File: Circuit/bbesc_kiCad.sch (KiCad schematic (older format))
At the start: 79 parts, among them J1 CONN_01X02, J10 CONN_01X01, J11 CONN_01X01, J12 CONN_01X01, J13 CONN_01X01, J14 CONN_01X01, J15 CONN_01X02, J16 CONN_01X02, J17 CONN_01X01, J18 CONN_01X01, J19 CONN_01X01, J2 CONN_01X06, J3 CONN_01X06, J4 CONN_01X06, J5 CONN_01X02, J6 CONN_01X02, J7 CONN_01X01, J8 CONN_01X01, J9 RJ45, Q1 Q_NMOS_GDS, Q2 Q_NMOS_GDS, Q3 Q_NMOS_GDS, Q4 Q_NMOS_GDS, Q5 Q_NMOS_GDS, Q6 Q_NMOS_GDS, U1 teensy_3-2, U2 IR2101, U3 IR2101, U4 IR2101, U5 LM324N, U6 LM7805

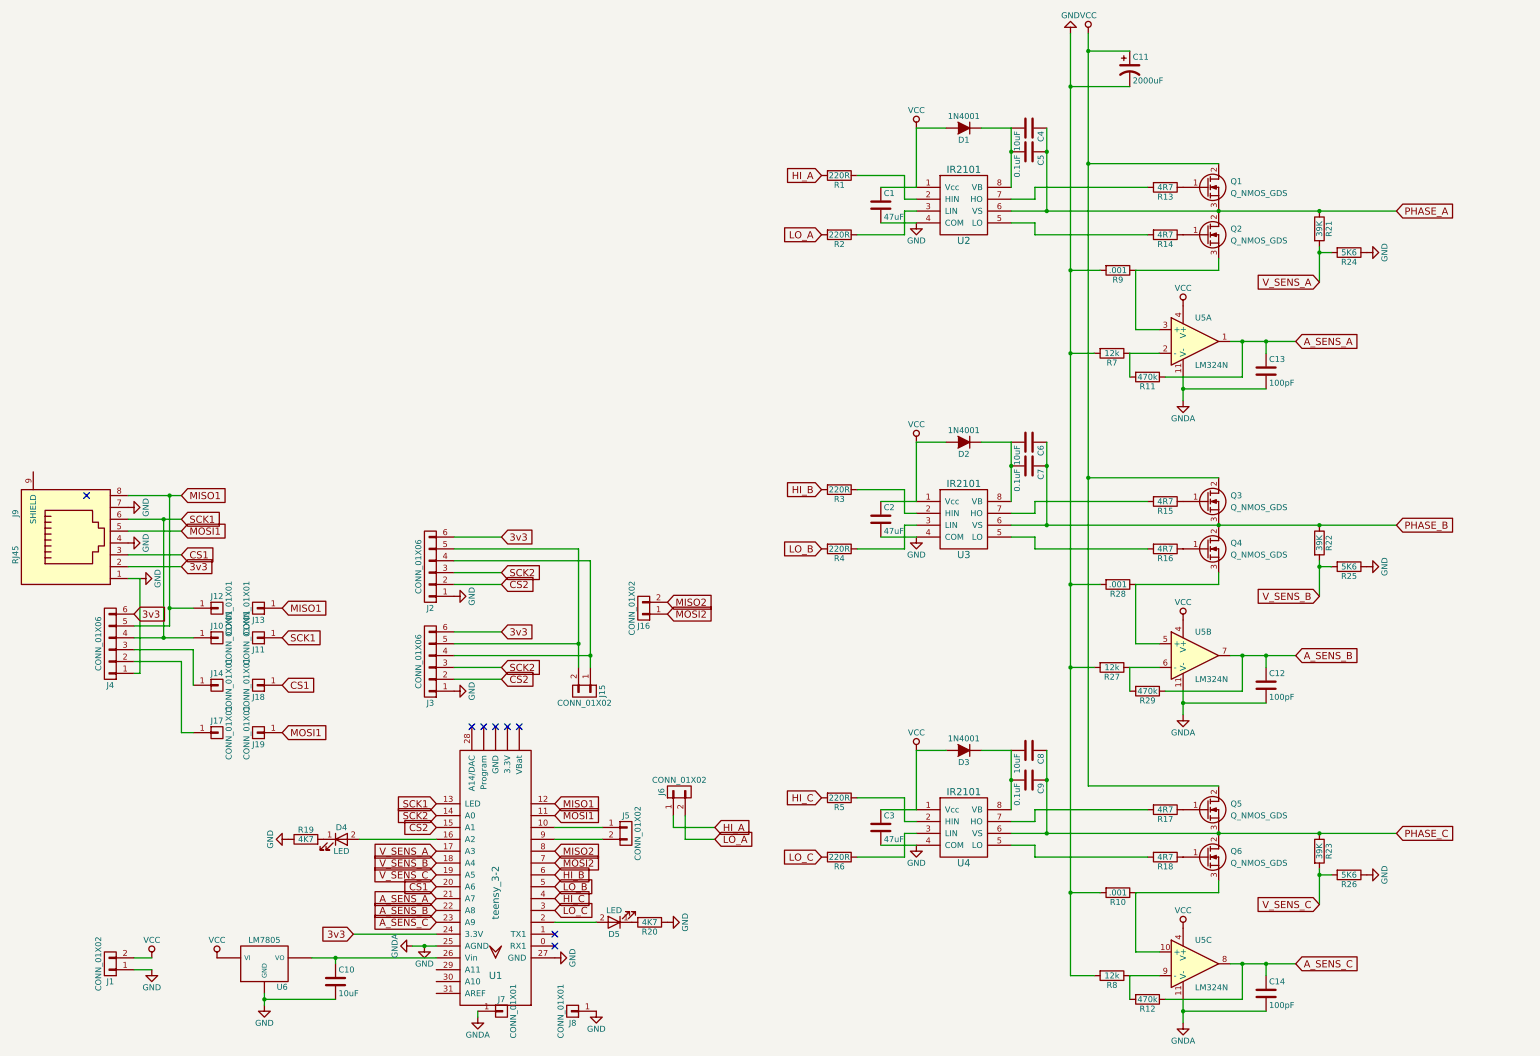
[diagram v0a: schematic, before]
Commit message: circuit for fab, foc bones
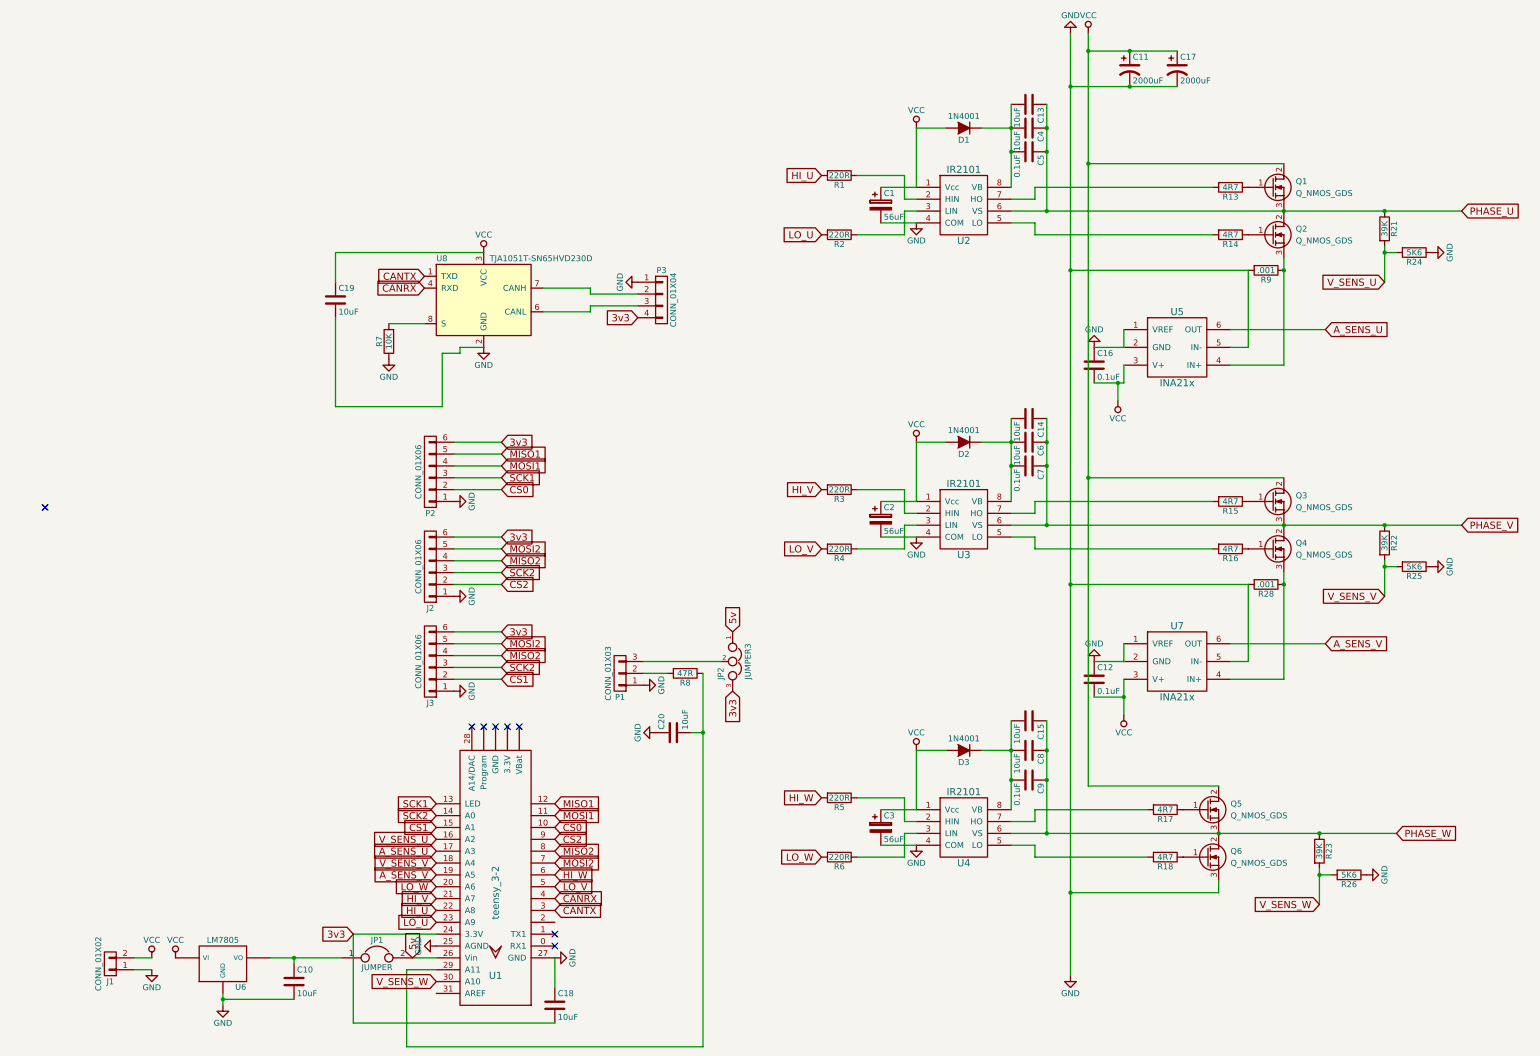
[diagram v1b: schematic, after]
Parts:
- removed C1, C2, C3: 47uF, Capacitors_SMD:C_1206_HandSoldering, symbol C
- removed D4, D5: LED, LEDs:LED_1206, symbol LED-RESCUE-bbesc_kiCad
- removed J10, J11, J12, J13, J14, J17, J18, J19, J7, J8: CONN_01X01, Pin_Headers:Pin_Header_Straight_1x01_Pitch2.54mm, symbol CONN_01X01
- removed J15, J16, J5, J6: CONN_01X02, Pin_Headers:Pin_Header_Straight_1x02_Pitch2.54mm, symbol CONN_01X02
- removed J4: CONN_01X06, Pin_Headers:Pin_Header_Straight_1x06_Pitch2.54mm, symbol CONN_01X06
- removed J9: RJ45, Connectors:RJ45_8, symbol RJ45
- removed R10: .001, R_SHUNT_3920:R_2816_HandSoldering, symbol R
- removed R11, R12, R29: 470k, Resistors_SMD:R_1206_HandSoldering, symbol R
- removed R19, R20: 4K7, Resistors_SMD:R_1206_HandSoldering, symbol R
- removed R27: 12k, Resistors_SMD:R_1206_HandSoldering, symbol R
- removed U5: LM324N, Housings_DIP:DIP-14_W7.62mm_Socket_LongPads, symbol LM324N
- added C1, C2, C3: 56uF, Capacitors_SMD:CP_Elec_6.3x7.7, symbol CP
- added C15, C18, C19, C20: 10uF, Capacitors_SMD:C_1206_HandSoldering, symbol C
- added C16: 0.1uF, Capacitors_SMD:C_1206_HandSoldering, symbol C
- added C17: 2000uF, Capacitors_ThroughHole:CP_Radial_D13.0mm_P5.00mm, symbol CP1
- added JP1: JUMPER, Pin_Headers:Pin_Header_Straight_1x02_Pitch2.54mm, symbol JUMPER
- added JP2: JUMPER3, Pin_Headers:Pin_Header_Straight_1x03_Pitch2.54mm, symbol JUMPER3
- added P1: CONN_01X03, Pin_Headers:Pin_Header_Straight_1x03_Pitch2.54mm, symbol CONN_01X03
- added P2: CONN_01X06, Pin_Headers:Pin_Header_Straight_1x06_Pitch2.54mm, symbol CONN_01X06
- added P3: CONN_01X04, Pin_Headers:Pin_Header_Straight_1x04_Pitch2.54mm, symbol CONN_01X04
- added U5, U7: INA21x, TO_SOT_Packages_SMD:SOT-363_SC-70-6_Handsoldering, symbol INA21x
- added U8: TJA1051T-SN65HVD230D, Housings_SOIC:SOIC-8_3.9x4.9mm_Pitch1.27mm, symbol TJA1051T
- C11: footprint Capacitors_THT:CP_Radial_D16.0mm_P7.50mm -> Capacitors_ThroughHole:CP_Radial_D13.0mm_P5.00mm
- C12: value 100pF -> 0.1uF
- C13, C14: value 100pF -> 10uF
- R7: value 12k -> 10K
- R8: value 12k -> 47R
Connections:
- net HI_A is gone; now on net HI_U: R1.2
- net LO_A is gone; now on net LO_U: R2.2
- net 3v3: now also C18.2, JP2.3, P2.6 (P6), P3.4 (P4)
- net CS1: now also J3.2 (P2), U1.15 (A1); no longer U1.20 (A6)
- net CS2: now also U1.9; no longer J3.2 (P2), U1.15 (A1)
- net GND: now also C12.1, Q6.3 (S), R7.1, C1.2, C16.1, C17.2, C18.1, C19.2, C2.2, C20.1, C3.2, P1.1 (P1), P2.1 (P1), P3.1 (P1), U5.1 (VREF), U5.2 (GND), U5.5 (IN-), U7.1 (VREF), U7.2 (GND), U7.5 (IN-), U8.2 (GND); no longer C12.2, C13.2, C14.2, R7.2, R8.2
- net MISO1: now also P2.5 (P5)
- net MISO2: now also J2.4 (P4), J3.4 (P4)
- net MOSI1: now also P2.4 (P4)
- net MOSI2: now also J2.5 (P5), J3.5 (P5)
- net SCK1: now also P2.3 (P3)
- net VCC: now also C12.2, C1.1, C16.2, C17.1, C19.1, C2.1, C3.1, U5.3 (V+), U7.3 (V+), U8.3 (VCC)
- net at C8.2, C9.2, D3.1 (K)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: now also C15.2
- net at R8.1: now also U1.29 (A11), C20.2
- net at Q4.3 (S), R28.1: now also U7.4 (IN+)
- net at C6.2, C7.2, D2.1 (K)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: now also C14.2
- net at Q2.3 (S), R9.1: now also U5.4 (IN+)
- net at C4.2, C5.2, D1.1 (K)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: now also C13.2
- net CS0: now reaches U1.10
- net CS0: now also P2.2 (P2)
- net V_SENS_U: now reaches U1.16 (A2)
- net V_SENS_U: now also R21.2, R24.2
- net at C10.1, U6.3 (VO): now also JP1.1; no longer U1.26 (Vin)
- net V_SENS_W: now reaches U1.30 (A10)
- net V_SENS_W: now also R23.2, R26.2
- net A_SENS_A renamed HI_V
- net HI_V: now also R3.2; no longer C13.1
- net A_SENS_B renamed HI_U
- net HI_U: no longer C12.1
- net A_SENS_C renamed LO_U
- net LO_U: no longer C14.1
- net HI_B renamed HI_W
- net HI_W: now also R5.2; no longer R3.2
- net HI_C renamed CANRX
- net CANRX: now also U8.4 (RXD); no longer R5.2
- net LO_B renamed LO_V
- net LO_C renamed CANTX
- net CANTX: now also U8.1 (TXD); no longer R6.2
- net PHASE_A renamed PHASE_U
- net PHASE_U: now also C13.1
- net PHASE_B renamed PHASE_V
- net PHASE_V: now also C14.1
- net PHASE_C renamed PHASE_W
- net PHASE_W: now also C15.1
- removed net V_SENS_A: R21.2, R24.2, U1.17 (A3)
- net V_SENS_B renamed V_SENS_V
- removed net V_SENS_C: R23.2, R26.2, U1.19 (A5)
- new net: P1.2 (P2), R8.2
- new net: JP2.2, P1.3 (P3)
- new net: P3.3 (P3), U8.6 (CANL)
- new net: P3.2 (P2), U8.7 (CANH)
- new net: R7.2, U8.8 (S)
- new net 5v: JP1.2, JP2.1, U1.26 (Vin)
- new net A_SENS_U: U1.17 (A3), U5.6 (OUT)
- new net A_SENS_V: U1.19 (A5), U7.6 (OUT)
- new net LO_W: R6.2, U1.20 (A6)
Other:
- moved on the sheet: C10, C12, Q1, Q2, Q3, Q4, R13, R14, R15, R16, R21, R22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

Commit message: board v0.2
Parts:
- removed C1, C2, C3: 56uF, Capacitors_SMD:CP_Elec_6.3x7.7, symbol CP
- removed C8: 10uF, Capacitors_SMD:C_1206_HandSoldering, symbol C
- removed D1, D3: 1N4001, Diodes_SMD:D_SMA_Handsoldering, symbol D
- removed R1, R2: 220R, Resistors_SMD:R_1206_HandSoldering, symbol R
- removed R22: 39K, Resistors_SMD:R_1206_HandSoldering, symbol R
- removed R28: .001, R_SHUNT_3920:R_2816_HandSoldering, symbol R
- removed U2, U3, U4: IR2101, Housings_DIP:DIP-8_W7.62mm_Socket_LongPads, symbol IR2101
- removed U5, U7: INA21x, TO_SOT_Packages_SMD:SOT-363_SC-70-6_Handsoldering, symbol INA21x
- removed U6: LM7805, TO_SOT_Packages_THT:TO-220_Horizontal, symbol LM7805-RESCUE-bbesc_kiCad
- added C11: 22nF, Capacitors_SMD:C_1206_HandSoldering, symbol C
- added C17: 100nF, Capacitors_SMD:C_1206_HandSoldering, symbol C
- added C18, C19, C20: 220nF, Capacitors_SMD:C_1206_HandSoldering, symbol C
- added C21, C22: 2.2nF, Capacitors_SMD:C_1206_HandSoldering, symbol C
- added C24: 100uF, Capacitors_SMD:CP_Elec_6.3x7.7, symbol CP1
- added C26, C27, C28, C29, C30, C31: 10uF, Capacitors_SMD:C_1206_HandSoldering, symbol C
- added D1: DIODESCH, Diodes_SMD:D_SMA_Handsoldering, symbol D_Schottky
- added JP2: JUMPER, Pin_Headers:Pin_Header_Straight_1x02_Pitch2.54mm, symbol JUMPER
- added L1: 22uH, Inductors:Inductor_Taiyo-Yuden_NR-40xx_HandSoldering, symbol INDUCTOR
- added P4: CONN_01X04, Pin_Headers:Pin_Header_Straight_1x04_Pitch2.54mm, symbol CONN_01X04
- added R10: 1M, Resistors_SMD:R_1206_HandSoldering, symbol R
- added R11, R12, R13, R14: 100R, Resistors_SMD:R_1206_HandSoldering, symbol R
- added R17, R29: 39k, Resistors_SMD:R_1206_HandSoldering, symbol R
- added R18, R24: SHNT, R_SHUNT_3920:R_SHUNT_3920, symbol SHNT
- added R30: 39K, Resistors_SMD:R_1206_HandSoldering, symbol R
- added R31: 5K6, Resistors_SMD:R_1206_HandSoldering, symbol R
- added R7: 3k3, Resistors_SMD:R_1206_HandSoldering, symbol R
- added R8: 15k, Resistors_SMD:R_1206_HandSoldering, symbol R
- added U3: DRV_8302, HTSSOP-56:TSSOP-56_6.1x14mm_Pitch0.5mm, symbol DRV_8302
- C10, C4: value 10uF -> 2.2uF
- C12, C16: value 0.1uF -> 10uF
- C5, C7: value 0.1uF -> 2.2uF
- C6: value 10uF -> 120pF
- C9: value 0.1uF -> 6.8nF
- D2: value 1N4001 -> TVS 5v
- Q1, Q2, Q3, Q4, Q5, Q6: footprint TO-251_IPAK_Slammed:TO-251_IPAK_Vertical -> HTO-252:TO-252-2
- R23: value 39K -> 39k
- R25: value 5K6 -> 39K
- R3: value 220R -> 18k
- R4, R6: value 220R -> 3k3
- R5: value 220R -> 10k
- R9: value .001 -> 220k; footprint R_SHUNT_3920:R_2816_HandSoldering -> Resistors_SMD:R_1206_HandSoldering
- renumbered C19 to C1, C18 to C2, C11 to C23, C17 to C25, C20 to C3, J2 to J1, J3 to J2, J1 to J3, JP2 to JP3, P2 to P1, P1 to P2, R7 to R1, R13 to R15, R14 to R16, R21 to R19, R8 to R2, R24 to R20, R15 to R21, R16 to R22, R17 to R27, R18 to R28, U8 to U1, U1 to U2
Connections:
- net 3v3: now also P4.4 (P4)
- net 5v: now also D2.1 (K), JP1.1, R3.2, R5.2, C24.1, L1.1; no longer JP1.2, U2.26 (Vin)
- net A_SENS_U: now also U3.25 (SO1)
- net A_SENS_V: now also U3.26 (SO2)
- net CS1: now also JP2.2; no longer U2.15 (A1)
- net GND: now also C12.2, C13.2, C14.2, C15.2, C4.2, C5.2, C6.2, C7.2, C9.2, D2.2 (A), Q2.3 (S), R20.2, R26.2, R4.1, R6.1, C24.2, C26.2, C27.2, C28.2, C29.2, C30.2, C31.2, D1.2 (A), P4.1 (P1), R10.1, R17.1, R18.2, R24.2, R31.2, R7.1, U3.28 (AGND), U3.44 (SL_A), U3.57 (GND); no longer C12.1, Q6.3 (S), R20.1, R25.1, R26.1
- net PHASE_U: now also C18.1, U3.46 (SH_A); no longer C13.1, C4.1, C5.1
- net PHASE_V: now also R25.1, C19.1, U3.41 (SH_B); no longer C14.1, C6.1, C7.1
- net PHASE_W: now also C20.1, R30.1, U3.36 (SH_C); no longer C15.1, C9.1, R23.1
- net VCC: now also C12.1, C13.1, C14.1, C15.1, C26.1, C27.1, C28.1, C29.1, C30.1, C31.1, U3.29 (PVDD1), U3.53 (PVDD2), U3.54 (PVDD2); no longer C12.2, D2.2 (A)
- net V_SENS_U: now also R20.1, U2.30 (A10); no longer R20.2, U2.16 (A2)
- net V_SENS_V: now also R26.1
- net V_SENS_W: now also U2.16 (A2), R30.2, R31.1; no longer R23.2, R26.2, U2.30 (A10)
- net at Q6.1 (G), R28.1: now also R29.2
- net at R5.1: now also U3.10 (GAIN), U3.9 (M_OC)
- net DRV_LO_W: now reaches R28.2
- net DRV_LO_W: now also U3.35 (GL_C)
- net DRV_HI_W: now reaches R27.2
- net DRV_HI_W: now also U3.37 (GH_C)
- net at Q4.1 (G), R22.1: now also R23.2
- net H_V_LO: now reaches Q4.3 (S)
- net H_V_LO: now also R23.1, R18.1, U3.39 (SL_B)
- net at R3.1: now also R4.2, U3.3 (VSENS)
- net DRV_LO_V: now reaches R22.2
- net DRV_LO_V: now also U3.40 (GL_B)
- net DRV_HI_V: now reaches R21.2
- net DRV_HI_V: now also U3.42 (GH_B)
- net at R9.1: now also U3.1 (RT_CLK); no longer Q2.3 (S)
- net at Q2.1 (G), R16.1: now also R17.2
- net DRV_LO_U: now reaches R16.2
- net DRV_LO_U: now also U3.45 (GL_A)
- net DRV_HI_U: now reaches R15.2
- net DRV_HI_U: now also U3.47 (GH_A)
- net EN_GATE: now reaches U2.2
- net EN_GATE: now also U3.16 (EN_GATE)
- net DRV_FAULT: now reaches U2.28 (A14/DAC)
- net DRV_FAULT: now also U3.6 (nFAULT)
- net SIMPLE_INPUT: now reaches C3.2, R2.1, U2.29 (A11)
- net MC_AREF: now reaches U2.31 (AREF)
- net MC_AREF: now also U3.24 (REF)
- net at C10.1: now also U3.27 (AVDD); no longer JP1.1
- net at P3.3 (P3), U1.6 (CANL): now also P4.3 (P3)
- net at P3.2 (P2), U1.7 (CANH): now also P4.2 (P2)
- net HI_U renamed MC_HI_U
- net MC_HI_U: now also U3.17 (INH_A)
- net HI_V renamed MC_HI_V
- net MC_HI_V: now also U3.19 (INH_B); no longer R3.2
- net HI_W renamed MC_HI_W
- net MC_HI_W: now also U3.21 (INH_C); no longer R5.2
- net LO_U renamed MC_LO_U
- net MC_LO_U: now also U3.18 (INL_A)
- net LO_V renamed MC_LO_V
- net MC_LO_V: now also U3.20 (INL_B); no longer R4.2
- net LO_W: no longer names the net of R6.2
- net LO_W: now also U3.7 (DTC); no longer U2.20 (A6)
- new net: JP1.2, U2.26 (Vin)
- new net: C4.1, C5.1, U3.11 (OC_ADJ), U3.23 (DVDD)
- new net: C7.1, U3.13 (GVDD)
- new net: C11.1, U3.14 (CP1)
- new net: C11.2, U3.15 (CP2)
- new net: C6.1, R8.1, U3.2 (COMP)
- new net: C22.1, R14.2, U3.30 (SP2)
- new net: C22.2, R13.2, U3.31 (SN2)
- new net: C21.1, R12.2, U3.32 (SP1)
- new net: C21.2, R11.2, U3.33 (SN1)
- new net: C20.2, U3.38 (BST_C)
- new net: C19.2, U3.43 (BST_B)
- new net: C18.2, U3.48 (BST_A)
- new net: R10.2, U3.49 (BIAS)
- new net: C17.1, D1.1 (K), L1.2, U3.50 (PH), U3.51 (PH)
- new net: C17.2, U3.52 (BST_BK)
- new net: R7.2, U3.8 (M_PWM)
- new net: C9.1, R8.2
- new net DC_CAL: JP2.1, U2.15 (A1), U3.12 (DC_CAL)
- new net H_W_LO: Q6.3 (S), R24.1, R29.1, U3.34 (SL_C)
- new net MC_LO_W: U2.20 (A6), U3.22 (INL_C)
- new net SHNT_V_HI: R13.1, R18.3
- new net SHNT_V_LO: R14.1, R18.4
- new net SHNT_W_HI: R11.1, R24.3
- new net SHNT_W_LO: R12.1, R24.4
- no-connect marks 8 -> 11
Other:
- moved on the sheet: C1, C2, C23, C25, C3, J1, J2, J3, JP1, JP3, P1, P2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
